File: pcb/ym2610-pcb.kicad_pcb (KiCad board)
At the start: 4 copper layers, 100.9 x 77.5 mm, 132 parts, among them J1 MIDI_IN, J2 LINE_OUT, J3 HEADPHONES, J4 SPDIF_COAX, J5 UART, SW1 BTN_A, SW2 BTN_B, SW3 CRESET, U1 YM2610, U10 TSV914IPT, U11 TSV914IPT, U12 AD8532, U13 74LVC2G08, U14 74AHCT595, U15 74AHCT595, U16 SPDIF_OPTICAL, U17 74HCT573, U18 TLP2361, U19 74HCT153, U2 YM3016, U20 74HCT153, U21 74LVC257, U3 74LV1T34, U4 74LVC244, U5 74LV1T34, U6 74HCT573, U7 74HCT573, U8 74HCT153, U9 74HCT153

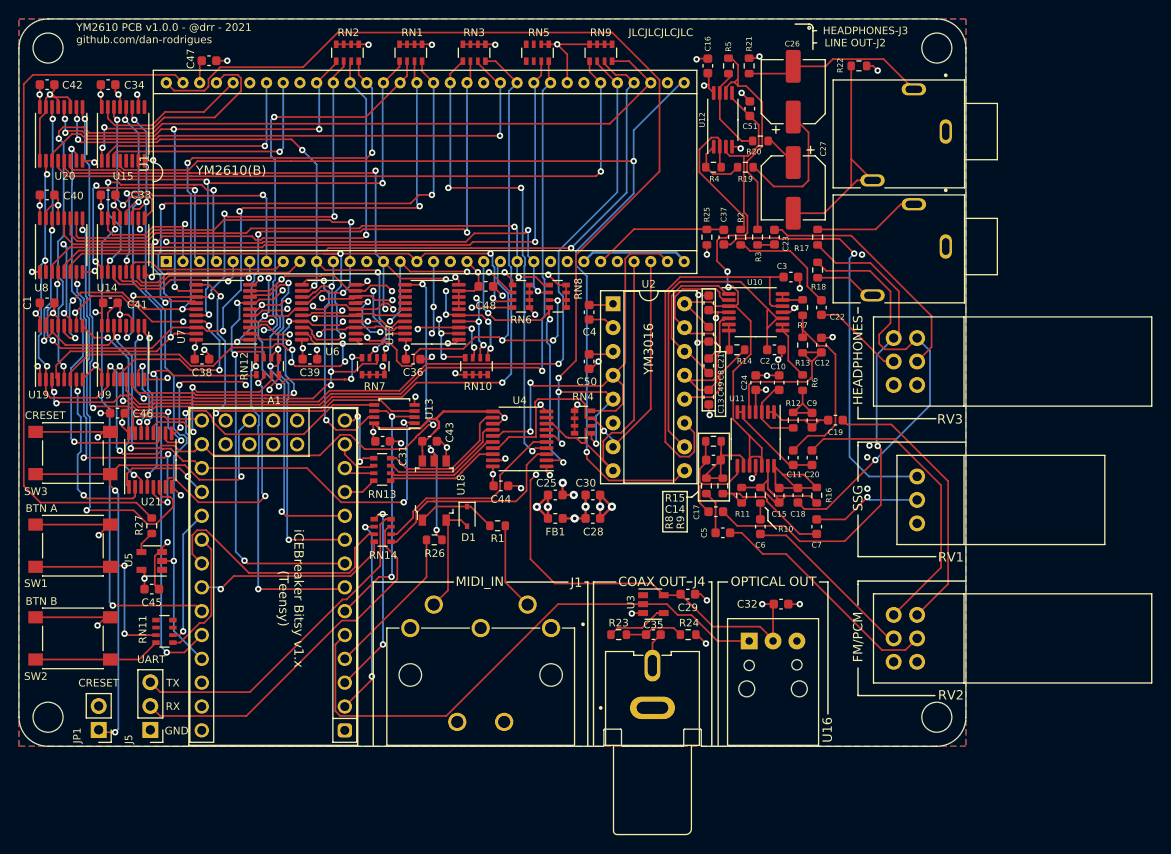
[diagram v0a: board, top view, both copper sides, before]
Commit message: 1.0.0 of PCB as pictured in repo
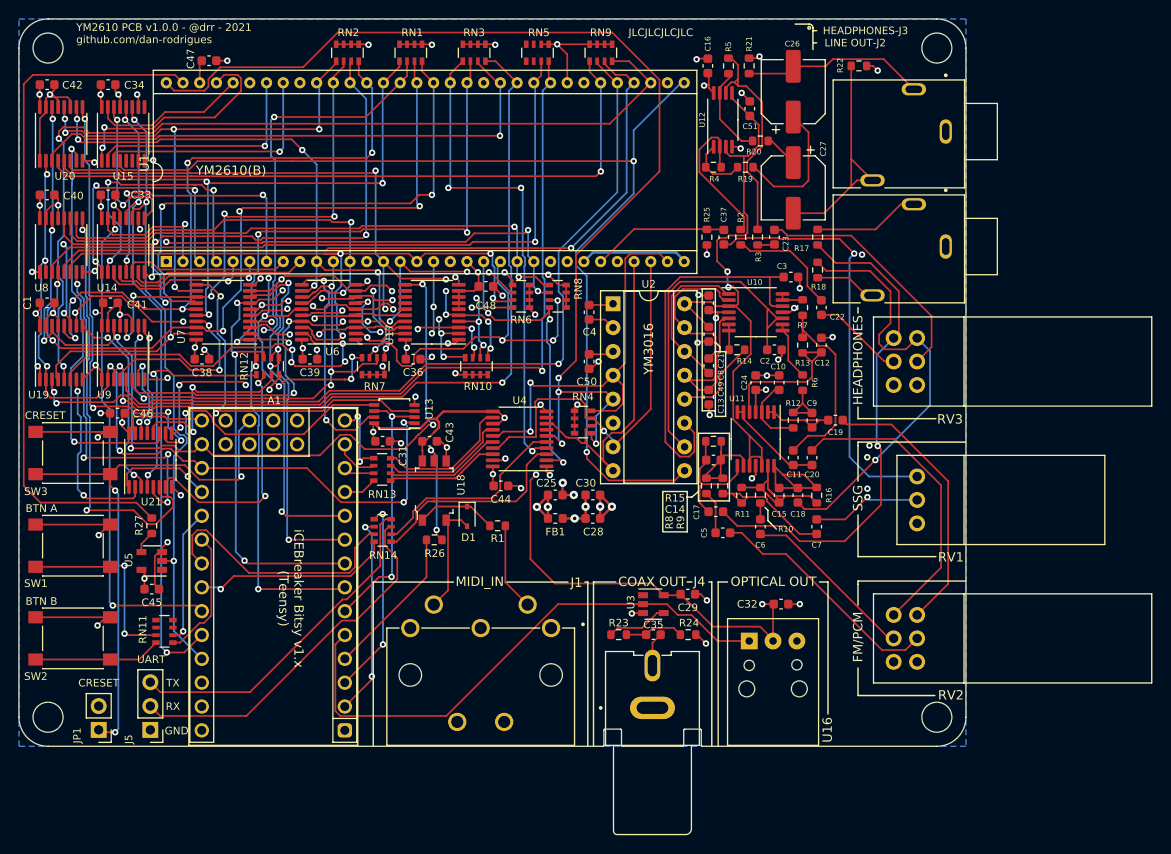
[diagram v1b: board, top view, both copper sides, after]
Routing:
- removed copper zone on F.Cu, net GND
